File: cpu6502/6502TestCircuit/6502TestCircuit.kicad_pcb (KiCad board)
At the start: 2 copper layers, 45.7 x 40.6 mm, 15 parts, among them J1 Power, J2 Power, J3 Reset, SW1 Reset, U6 L7805, U9 DS1813

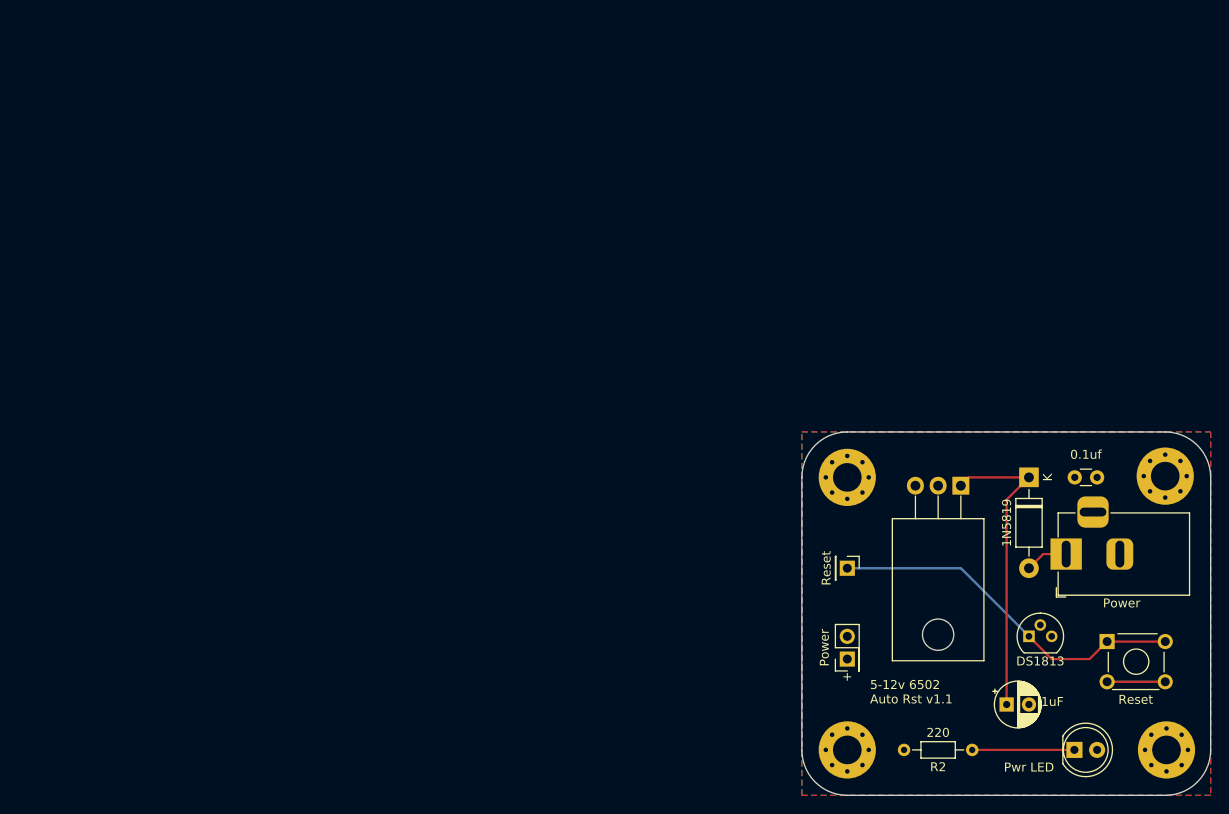
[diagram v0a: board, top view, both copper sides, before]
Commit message: code changes (wip), set test PCB 2.0 to PCBway
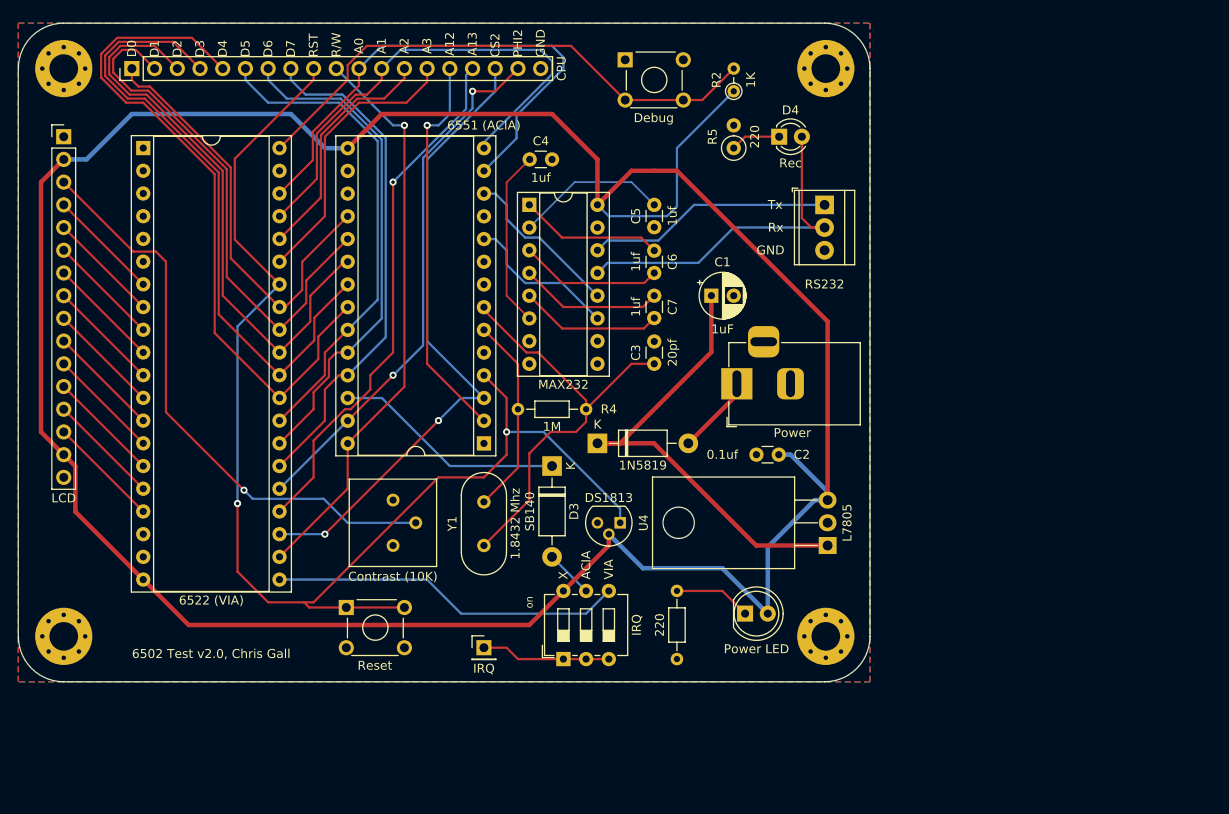
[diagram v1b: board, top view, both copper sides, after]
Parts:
- removed C8: 0.1uf, Capacitor_THT:C_Disc_D3.0mm_W1.6mm_P2.50mm
- removed SW1: Reset, Button_Switch_THT:SW_TH_Tactile_Omron_B3F-10xx
- removed U6: L7805, Package_TO_SOT_THT:TO-220-3_Horizontal_TabDown
- added C1: 1uF, Capacitor_THT:CP_Radial_D5.0mm_P2.50mm, F.Cu at (106.7, 53.3)
- added C2: 0.1uf, Capacitor_THT:C_Disc_D3.0mm_W1.6mm_P2.50mm, F.Cu at (114.3, 71.1)
- added C3: 20pf, Capacitor_THT:C_Disc_D3.0mm_W1.6mm_P2.50mm, F.Cu at (100.3, 61.0)
- added C4: 1uf, Capacitor_THT:C_Disc_D3.0mm_W1.6mm_P2.50mm, F.Cu at (86.4, 38.1)
- added C5: 1uf, Capacitor_THT:C_Disc_D3.0mm_W1.6mm_P2.50mm, F.Cu at (100.3, 45.7)
- added C6: 1uf, Capacitor_THT:C_Disc_D3.0mm_W1.6mm_P2.50mm, F.Cu at (100.3, 48.3)
- added D2: Power LED, LED_THT:LED_D5.0mm, F.Cu at (110.5, 88.9)
- added D4: Rec, LED_THT:LED_D3.0mm, F.Cu at (114.3, 35.6)
- added J4: Power, Connector_BarrelJack:BarrelJack_Horizontal, F.Cu at (109.6, 63.2)
- added J5: RS232, TerminalBlock_TE-Connectivity:TerminalBlock_TE_282834-3_1x03_P2.54mm_Horizontal, F.Cu at (119.4, 43.2)
- added R3: 220, Resistor_THT:R_Axial_DIN0204_L3.6mm_D1.6mm_P7.62mm_Horizontal, F.Cu at (102.9, 86.4)
- added R4: 1M, Resistor_THT:R_Axial_DIN0204_L3.6mm_D1.6mm_P7.62mm_Horizontal, F.Cu at (92.7, 66.0)
- added R5: 220, Resistor_THT:R_Axial_DIN0207_L6.3mm_D2.5mm_P2.54mm_Vertical, F.Cu at (109.2, 36.8)
- added RV2: Contrast (10K), Potentiometer_THT:Potentiometer_Bourns_3386P_Vertical, F.Cu at (71.1, 81.3)
- added SW2: Debug, Button_Switch_THT:SW_TH_Tactile_Omron_B3F-10xx, F.Cu at (97.1, 27.0)
- added SW3: Reset, Button_Switch_THT:SW_TH_Tactile_Omron_B3F-10xx, F.Cu at (65.9, 88.2)
- added SW4: IRQ, Button_Switch_THT:SW_DIP_SPSTx03_Slide_6.7x9.18mm_W7.62mm_P2.54mm_LowProfile, F.Cu at (90.2, 94.0)
- added U1: 6522 (VIA), Package_DIP:DIP-40_W15.24mm_Socket, F.Cu at (43.2, 36.8)
- added U4: L7805, Package_TO_SOT_THT:TO-220-3_Horizontal_TabDown, F.Cu at (119.7, 81.3)
- added U5: DS1813, Package_TO_SOT_THT:TO-92, F.Cu at (96.5, 78.7)
- added U8: MAX232, Package_DIP:DIP-16_W7.62mm_Socket, F.Cu at (86.4, 43.2)
- added Y1: 1.8432 Mhz, Crystal:Crystal_HC49-4H_Vertical, F.Cu at (81.3, 81.3)
- C7: value 1uF -> 1uf; footprint Capacitor_THT:CP_Radial_D5.0mm_P2.50mm -> Capacitor_THT:C_Disc_D3.0mm_W1.6mm_P2.50mm
- D1: value Pwr LED -> 1N5819; footprint LED_THT:LED_D5.0mm -> Diode_THT:D_DO-41_SOD81_P10.16mm_Horizontal
- D3: value 1N5819 -> SB140
- J1: value Power -> CPU; footprint Connector_BarrelJack:BarrelJack_Horizontal -> Connector_PinHeader_2.54mm:PinHeader_1x19_P2.54mm_Vertical
- J2: value Power -> IRQ; footprint Connector_PinHeader_2.54mm:PinHeader_2x01_P2.54mm_Vertical -> Connector_PinHeader_2.54mm:PinHeader_1x01_P2.54mm_Vertical
- J3: value Reset -> LCD; footprint Connector_PinHeader_2.54mm:PinHeader_1x01_P2.54mm_Vertical -> Connector_PinHeader_2.54mm:PinHeader_1x16_P2.54mm_Vertical
- R2: value 220 -> 1K; footprint Resistor_THT:R_Axial_DIN0204_L3.6mm_D1.6mm_P7.62mm_Horizontal -> Resistor_THT:R_Axial_DIN0204_L3.6mm_D1.6mm_P2.54mm_Vertical
- U9: value DS1813 -> 6551 (ACIA); footprint Package_TO_SOT_THT:TO-92 -> Package_DIP:DIP-28_W15.24mm_Socket
- moved H3 145.0 mm to (34.3, 27.9)
- moved H2 124.5 mm to (34.3, 91.4)
- moved J1 117.8 mm to (41.9, 27.9), turned to 90 degrees
- moved J3 100.0 mm to (34.3, 35.6), turned to 0 degrees
- moved R2 78.3 mm to (109.2, 30.5), turned to 90 degrees
- moved H4 76.2 mm to (119.5, 27.9)
- moved U9 64.7 mm to (81.3, 69.9), turned to 180 degrees
- moved D1 63.4 mm to (94.0, 69.8)
- moved C7 60.4 mm to (100.3, 53.3), turned to -90 degrees
- moved D3 53.4 mm to (88.9, 72.4)
- moved J2 40.7 mm to (81.3, 92.7), turned to 0 degrees
- moved H1 17.9 mm to (119.5, 91.4)
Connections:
- C7 pad 1: Net-(D3-K) -> Net-(U8-C2+)
- C7 pad 2: GND -> Net-(U8-C2-)
- D1 pad 2: +5V -> Net-(D1-A)
- D3 pad 2: Net-(D3-A) -> /ACIAIRQ
- J1 pad 1: Net-(D3-A) -> /D0
- J1 pad 2: GND -> /D1
- J1 pad 3: (no net) -> /D2
- J2 pad 1: +5V -> /IRQ
- J3 pad 1: /RST -> GND
- R2 pad 1: Net-(D1-K) -> +5V
- R2 pad 2: GND -> /CA1
- U9 pad 1: /RST -> GND
- U9 pad 2: +5V -> /A12
- U9 pad 3: GND -> /CS2
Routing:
- net +5V: track 0.00 -> 309.6 mm
- net /RST: track 40.6 -> 141.5 mm, vias 0 -> 2
- net /D4: track 0.00 -> 76.9 mm
- net /CS2: track 0.00 -> 71.8 mm, vias 0 -> 2
- net /D3: track 0.00 -> 70.7 mm
- net Net-(J3-Pin_3): track 0.00 -> 65.0 mm, vias 0 -> 1
- net /D2: track 0.00 -> 64.7 mm
- net /R/W: track 0.00 -> 64.3 mm, vias 0 -> 1
- net /CA1: track 0.00 -> 60.5 mm
- net /PHI2: track 0.00 -> 59.5 mm, vias 0 -> 2
- net /A13: track 0.00 -> 58.9 mm, vias 0 -> 1
- net /A0: track 0.00 -> 58.5 mm
- net /D1: track 0.00 -> 58.3 mm
- net /D7: track 0.00 -> 56.8 mm
- net /D6: track 0.00 -> 56.2 mm
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- added copper zone on B.Cu, net GND
- removed copper zone on B.Cu, net +5V
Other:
- board size 45.7 x 40.6 mm -> 95.2 x 73.7 mm
- board text added: "6502 Test v2.0, Chris Gall"
- board text added: "A0"
- board text added: "A1"
- board text added: "A12"
- board text added: "A13"
- board text added: "A2"
- board text added: "A3"
- board text added: "ACIA"
- board text added: "CS2"
- board text added: "D0"
- board text added: "D1"
- board text added: "D2"
- board text added: "D3"
- board text added: "D4"
- board text added: "D5"
- board text added: "D6"
- board text added: "D7"
- board text added: "GND"
- board text added: "PHI2"
- board text added: "R/W"
- board text added: "RST"
- board text added: "Rx"
- board text added: "Tx"
- board text added: "VIA"
- board text added: "X"
- board text removed: "+"
- board text removed: "5-12v 6502 Auto Rst v1.1"
